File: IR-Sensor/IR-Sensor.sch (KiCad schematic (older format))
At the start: 11 parts, among them J1 Conn_01x03_Male, U1 LM324

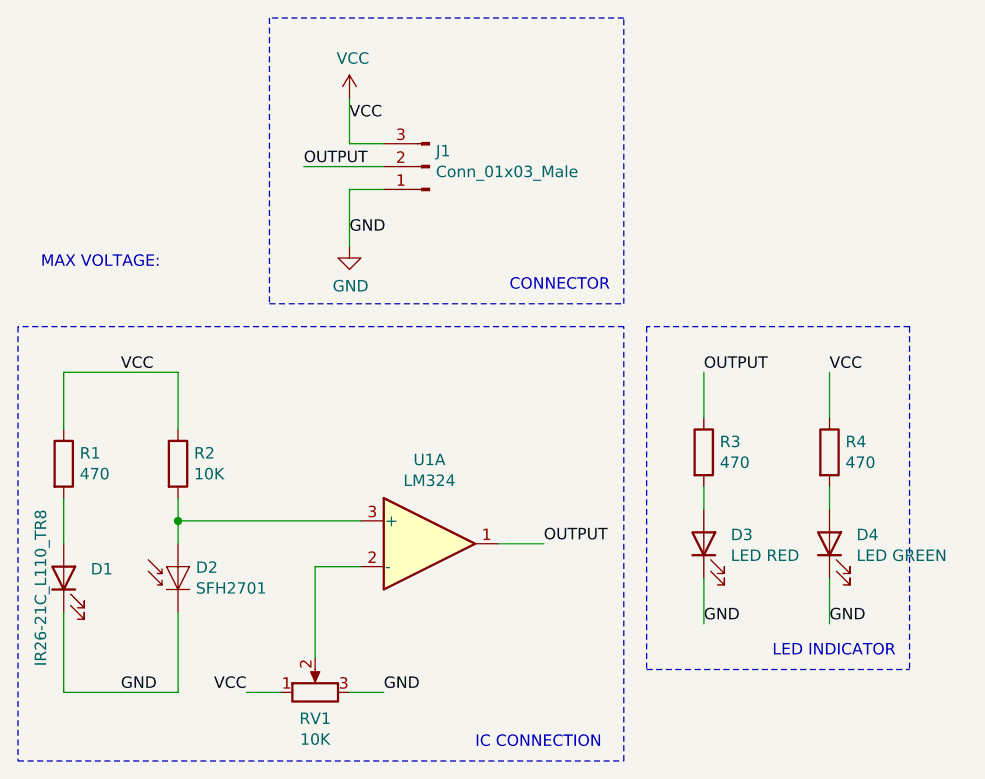
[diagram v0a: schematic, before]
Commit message: First commit in PCB layout
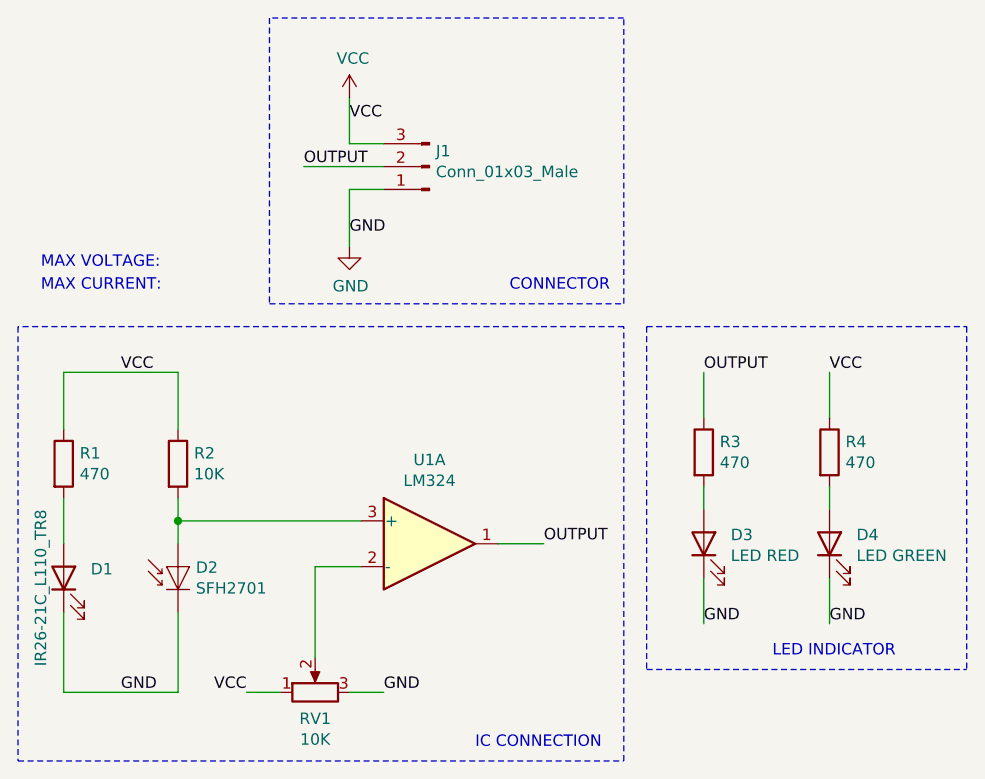
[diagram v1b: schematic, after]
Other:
- note added: "MAX CURRENT:"
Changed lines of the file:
@@
 Wire Notes Line
 	6650 2000 5100 2000
-Wire Notes Line
-	6750 4850 7900 4850
-Wire Notes Line
-	7900 3350 6750 3350
 Text Notes 6000 5200 0    50   ~ 0
 IC CONNECTION
@@
 LED INDICATOR
 Wire Notes Line
-	7900 3350 7900 4850
+	8150 3350 8150 4850
 Wire Notes Line
 	6750 3350 6750 4850
 Text Notes 4100 3100 0    50   ~ 0
 MAX VOLTAGE:
+Text Notes 4100 3200 0    50   ~ 0
+MAX CURRENT:
+Wire Notes Line
+	6750 4850 8150 4850
+Wire Notes Line
+	6750 3350 8150 3350
 $EndSCHEMATC
